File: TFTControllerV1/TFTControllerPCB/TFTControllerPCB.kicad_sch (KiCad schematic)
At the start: 17 parts, among them J1 Conn_01x40, J2 Conn_02x04_Counter_Clockwise, J3 Conn_02x04_Counter_Clockwise, J4 Conn_02x03_Counter_Clockwise, J5 Conn_02x03_Counter_Clockwise, Q1 BSS138, Q2 BSS138, SW1 SW_Push, U1 STM32F107VCTx, U2 XPT2046TS

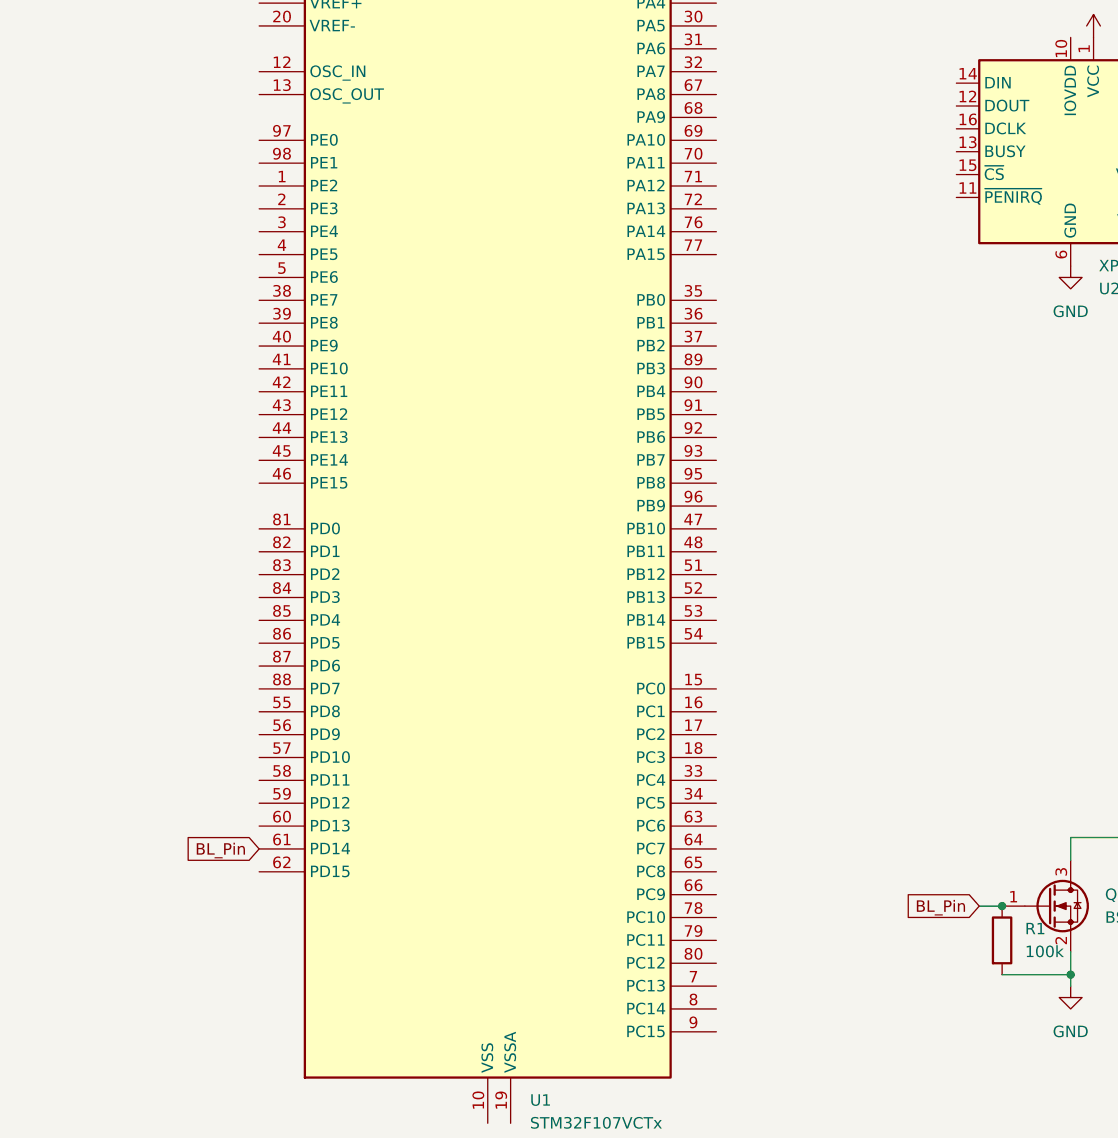
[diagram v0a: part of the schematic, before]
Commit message: working touch
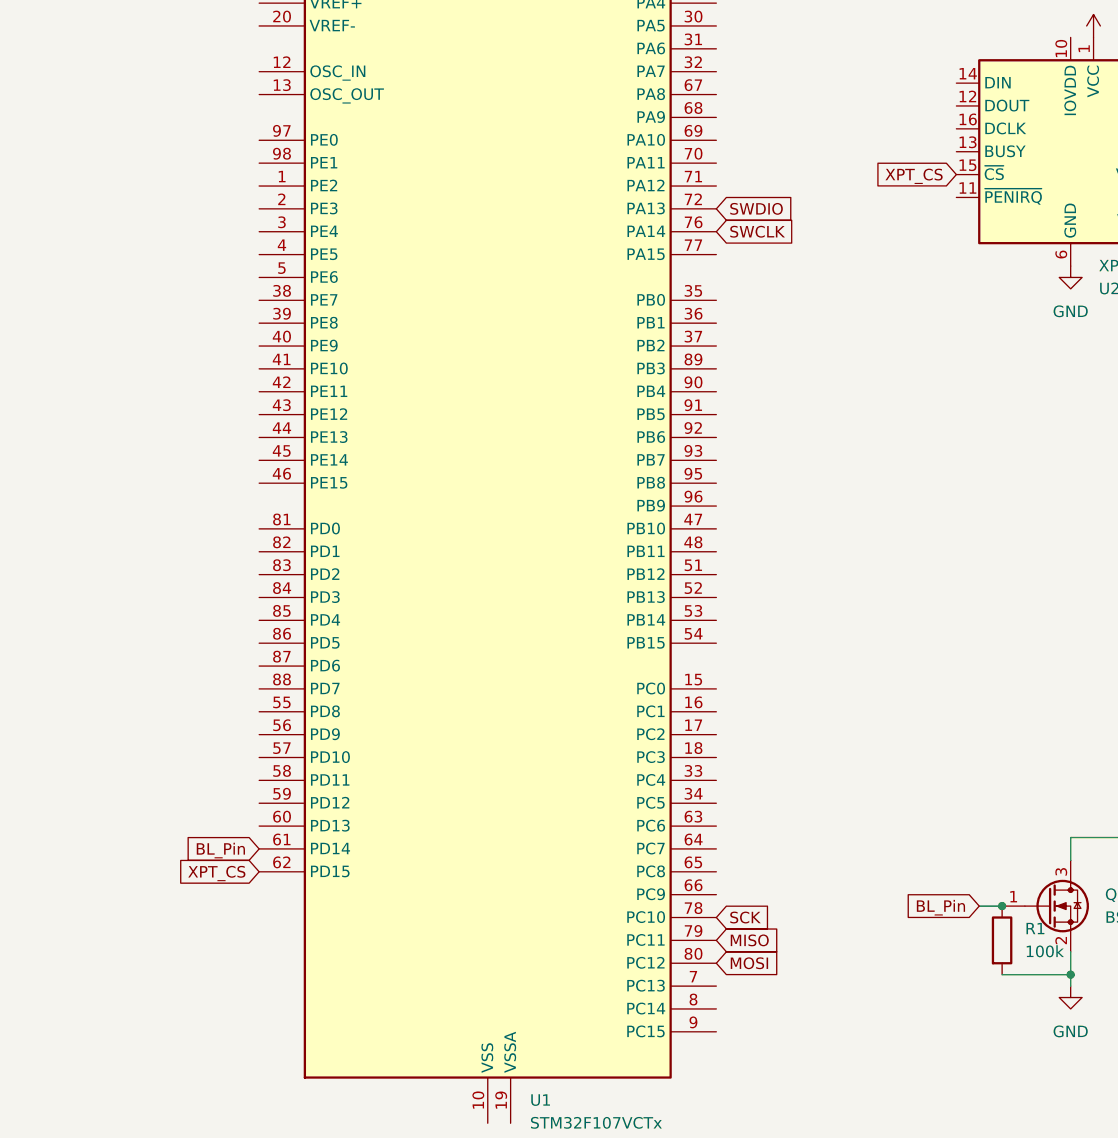
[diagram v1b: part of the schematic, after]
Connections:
- net XPT_CS: now reaches U2.15 (~{CS})
- net XPT_CS: now also U1.62 (PD15)
- net SWDIO: now reaches U1.72 (PA13)
- net SWCLK: now reaches U1.76 (PA14)
- net SCK: now reaches U1.78 (PC10)
- net MISO: now reaches U1.79 (PC11)
- net MOSI: now reaches U1.80 (PC12)
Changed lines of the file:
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@@
+		)
+	)
+	(global_label "XPT_CS"
+		(shape input)
+		(at 163.83 170.18 180)
+		(fields_autoplaced yes)
+		(effects
+			(font
+				(size 1.27 1.27)
+			)
+			(justify right)
+		)
+		(property "Intersheetrefs" "${INTERSHEET_REFS}"
+			(at 153.9506 170.18 0)
+			(effects
+				(font
+					(size 1.27 1.27)
+				)
+				(justify right)
+				(hide yes)
+			)
+		)
+	)
+	(global_label "MOSI"
+		(shape input)
+		(at 214.63 180.34 0)
+		(fields_autoplaced yes)
+		(effects
+			(font
+				(size 1.27 1.27)
+			)
+			(justify left)
+		)
+		(property "Intersheetrefs" "${INTERSHEET_REFS}"
+			(at 222.2114 180.34 0)
+			(effects
+				(font
+					(size 1.27 1.27)
+				)
+				(justify left)
+				(hide yes)
+			)
+		)
+	)
+	(global_label "MISO"
+		(shape input)
+		(at 214.63 177.8 0)
+		(fields_autoplaced yes)
+		(effects
+			(font
+				(size 1.27 1.27)
+			)
+			(justify left)
+		)
+		(property "Intersheetrefs" "${INTERSHEET_REFS}"
+			(at 222.2114 177.8 0)
+			(effects
+				(font
+					(size 1.27 1.27)
+				)
+				(justify left)
+				(hide yes)
+			)
+		)
+	)
+	(global_label "SWDIO"
+		(shape input)
+		(at 214.63 96.52 0)
+		(fields_autoplaced yes)
+		(effects
+			(font
+				(size 1.27 1.27)
+			)
+			(justify left)
+		)
+		(property "Intersheetrefs" "${INTERSHEET_REFS}"
+			(at 223.4814 96.52 0)
+			(effects
+				(font
+					(size 1.27 1.27)
+				)
+				(justify left)
+				(hide yes)
+			)
+		)
+	)
+	(global_label "SCK"
+		(shape input)
+		(at 214.63 175.26 0)
+		(fields_autoplaced yes)
+		(effects
+			(font
+				(size 1.27 1.27)
+			)
+			(justify left)
+		)
+		(property "Intersheetrefs" "${INTERSHEET_REFS}"
+			(at 221.3647 175.26 0)
+			(effects
+				(font
+					(size 1.27 1.27)
+				)
+				(justify left)
+				(hide yes)
+			)
+		)
+	)
+	(global_label "SWCLK"
+		(shape input)
+		(at 214.63 99.06 0)
+		(fields_autoplaced yes)
+		(effects
+			(font
+				(size 1.27 1.27)
+			)
+			(justify left)
+		)
+		(property "Intersheetrefs" "${INTERSHEET_REFS}"
+			(at 223.8442 99.06 0)
+			(effects
+				(font
+					(size 1.27 1.27)
+				)
+				(justify left)
+				(hide yes)
+			)
+		)
+	)
+	(global_label "XPT_CS"
+		(shape input)
+		(at 241.3 92.71 180)
+		(fields_autoplaced yes)
+		(effects
+			(font
+				(size 1.27 1.27)
+			)
+			(justify right)
+		)
+		(property "Intersheetrefs" "${INTERSHEET_REFS}"
+			(at 231.4206 92.71 0)
+			(effects
+				(font
+					(size 1.27 1.27)
+				)
+				(justify right)
+				(hide yes)
+			)
 		)
 	)
